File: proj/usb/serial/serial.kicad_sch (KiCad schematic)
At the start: 8 parts, among them J2 Conn_02x03_Odd_Even, Q1 BSS138, Q2 BSS138, U1 CH340K

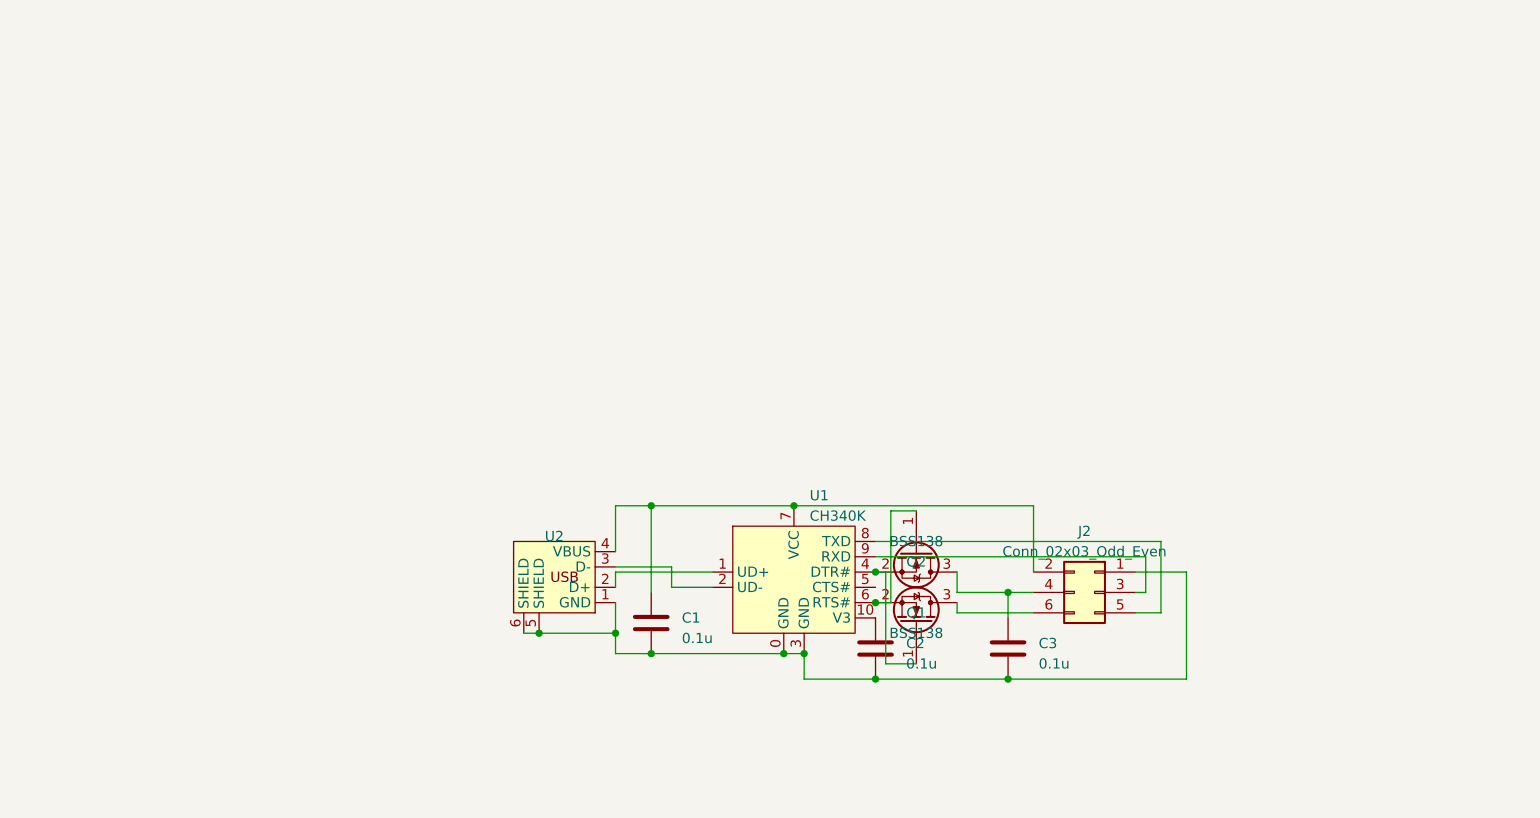
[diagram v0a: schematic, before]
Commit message: -
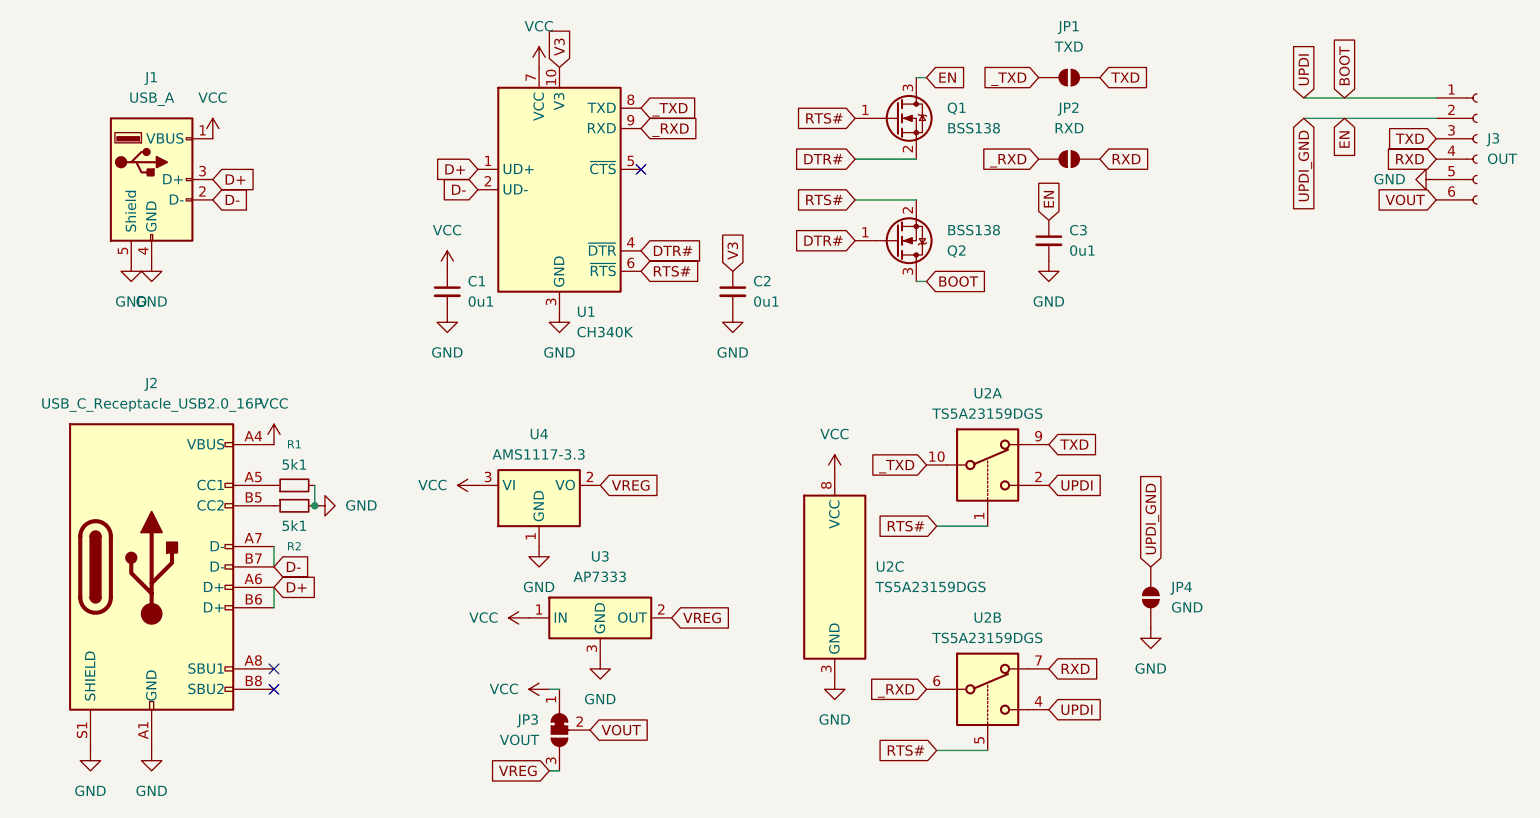
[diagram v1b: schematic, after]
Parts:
- removed C1, C2, C3: 0.1u, Capacitor_SMD:C_0603_1608Metric, symbol Device:C
- removed J2: Conn_02x03_Odd_Even, Connector_PinSocket_2.54mm:PinSocket_2x03_P2.54mm_Vertical, symbol Connector_Generic:Conn_02x03_Odd_Even
- removed U1: CH340K, Package_SO:SSOP-10_3.9x4.9mm_P1.00mm, symbol akizuki:CH340K
- removed U2: ~, Library:PCB_USB_Conn, symbol usb_a_pcb:PCB_USB_Conn
- added C1, C2, C3: 0u1, symbol Device:C_Small
- added J1: USB_A, symbol Connector:USB_A
- added J2: USB_C_Receptacle_USB2.0_16P, symbol Connector:USB_C_Receptacle_USB2.0_16P
- added J3: OUT, Connector_PinSocket_2.54mm:PinSocket_1x06_P2.54mm_Vertical, symbol Connector:Conn_01x06_Socket
- added JP1: TXD, Jumper:SolderJumper-2_P1.3mm_Open_RoundedPad1.0x1.5mm, symbol Jumper:SolderJumper_2_Open
- added JP2: RXD, Jumper:SolderJumper-2_P1.3mm_Open_RoundedPad1.0x1.5mm, symbol Jumper:SolderJumper_2_Open
- added JP3: VOUT, symbol Jumper:SolderJumper_3_Bridged12
- added JP4: GND, Jumper:SolderJumper-2_P1.3mm_Open_RoundedPad1.0x1.5mm, symbol Jumper:SolderJumper_2_Open
- added R1, R2: 5k1, symbol Device:R_Small
- added U1: CH340K, Package_SO:SSOP-10-1EP_3.9x4.9mm_P1mm_EP2.1x3.3mm, symbol Interface_USB:CH340K
- added U2: TS5A23159DGS, Package_SO:VSSOP-10_3x3mm_P0.5mm, symbol Analog_Switch:TS5A23159DGS
- added U3: AP7333, Package_TO_SOT_SMD:SOT-23-3, symbol Library:AP7333
- added U4: AMS1117-3.3, Package_TO_SOT_SMD:SOT-223-3_TabPin2, symbol Regulator_Linear:AMS1117-3.3
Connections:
- net DTR#: now reaches Q1.2 (S), Q2.1 (G)
- net DTR#: now also U1.4 (~{DTR})
- net RTS#: now reaches Q1.1 (G), Q2.2 (S)
- net RTS#: now also U1.6 (~{RTS}), U2.1, U2.5
- net EN: now reaches Q1.3 (D)
- net EN: now also C3.1, J3.2 (Pin_2), JP4.2 (B)
- net BOOT: now reaches Q2.3 (D)
- net BOOT: now also J3.1 (Pin_1), U2.2, U2.4
- new net: J2.A5 (CC1), R1.1
- new net: J2.B5 (CC2), R2.1
- new net D+: J1.3 (D+), J2.A6 (D+), J2.B6 (D+), U1.1 (UD+)
- new net D-: J1.2 (D-), J2.A7 (D-), J2.B7 (D-), U1.2 (UD-)
- new net GND: C1.2, C2.2, C3.2, J1.4 (GND), J1.5 (Shield), J2.A1 (GND), J2.A12 (GND), J2.B1 (GND), J2.B12 (GND), J2.S1 (SHIELD), J3.5 (Pin_5), JP4.1 (A), R1.2, R2.2, U1.11 (GND), U1.3 (GND), U2.3 (GND), U3.3 (GND), U4.1 (GND)
- new net RXD: J3.4 (Pin_4), JP2.2 (B), U2.7
- new net TXD: J3.3 (Pin_3), JP1.2 (B), U2.9
- new net V3: C2.1, U1.10 (V3)
- new net VCC: C1.1, J1.1 (VBUS), J2.A4 (VBUS), J2.A9 (VBUS), J2.B4 (VBUS), J2.B9 (VBUS), JP3.1 (A), U1.7 (VCC), U2.8 (VCC), U3.1 (IN), U4.3 (VI)
- new net VOUT: J3.6 (Pin_6), JP3.2 (C)
- new net VREG: JP3.3 (B), U3.2 (OUT), U4.2 (VO)
- new net _RXD: JP2.1 (A), U1.9 (RXD), U2.6
- new net _TXD: JP1.1 (A), U1.8 (TXD), U2.10
- no-connect marks 0 -> 3
